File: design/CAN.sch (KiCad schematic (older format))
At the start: 4 parts, among them U4 TJA1051TK3

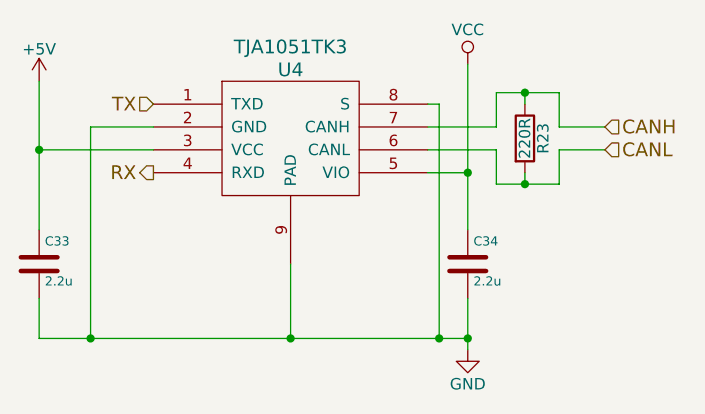
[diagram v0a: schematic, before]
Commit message: initial commit
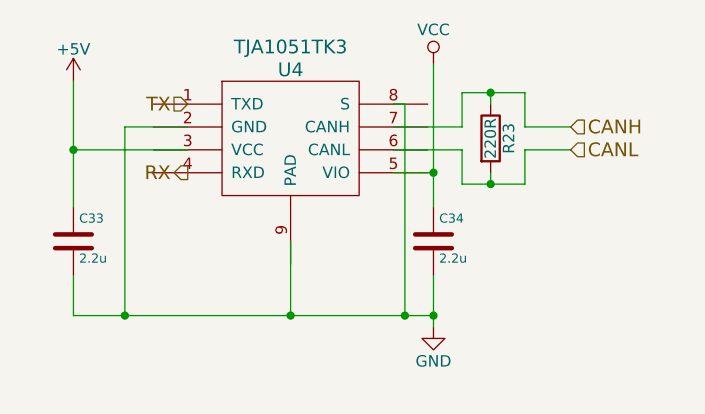
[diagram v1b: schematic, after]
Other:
- moved on the sheet: C33, C34, R23
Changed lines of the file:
@@
 LIBS:valves
 LIBS:crf_1
+LIBS:crf_2
 LIBS:VESC_6-cache
 EELAYER 25 0
@@
 L C C33
 U 1 1 53F59FA3
-P 4900 4550
-F 0 "C33" H 4925 4650 40  0000 L CNN
-F 1 "2.2u" H 4925 4475 40  0000 L CNN
-F 2 "CRF1:SMD-0603_c" H 4938 4400 30  0001 C CNN
-F 3 "" H 4900 4550 60  0000 C CNN
-	1    4900 4550
+P 5050 4450
+F 0 "C33" H 5075 4550 40  0000 L CNN
+F 1 "2.2u" H 5075 4375 40  0000 L CNN
+F 2 "CRF1:SMD-0603_c" H 5088 4300 30  0001 C CNN
+F 3 "" H 5050 4450 60  0000 C CNN
+	1    5050 4450
 	1    0    0    -1
 $EndComp
-Text HLabel 5400 4150 0    60   Output ~ 0
+Text HLabel 5550 4150 0    60   Output ~ 0
 RX
-Text HLabel 5400 3850 0    60   Input ~ 0
+Text HLabel 5550 3850 0    60   Input ~ 0
 TX
-Text HLabel 7375 3950 2    60   Input ~ 0
+Text HLabel 7225 3950 2    60   Input ~ 0
 CANH
-Text HLabel 7375 4050 2    60   Input ~ 0
+Text HLabel 7225 4050 2    60   Input ~ 0
 CANL
 $Comp
@@
 L C C34
 U 1 1 5A8B2DCC
-P 6775 4550
-F 0 "C34" H 6800 4650 40  0000 L CNN
-F 1 "2.2u" H 6800 4475 40  0000 L CNN
-F 2 "CRF1:SMD-0603_c" H 6813 4400 30  0001 C CNN
-F 3 "" H 6775 4550 60  0000 C CNN
-	1    6775 4550
+P 6625 4450
+F 0 "C34" H 6650 4550 40  0000 L CNN
+F 1 "2.2u" H 6650 4375 40  0000 L CNN
+F 2 "CRF1:SMD-0603_c" H 6663 4300 30  0001 C CNN
+F 3 "" H 6625 4450 60  0000 C CNN
+	1    6625 4450
 	1    0    0    -1
 $EndComp
@@
 L +5V #PWR063
 U 1 1 5A8B3017
-P 4900 3750
-F 0 "#PWR063" H 4900 3600 50  0001 C CNN
-F 1 "+5V" H 4900 3890 50  0000 C CNN
-F 2 "" H 4900 3750 50  0001 C CNN
-F 3 "" H 4900 3750 50  0001 C CNN
-	1    4900 3750
+P 5050 3750
+F 0 "#PWR063" H 5050 3600 50  0001 C CNN
+F 1 "+5V" H 5050 3890 50  0000 C CNN
+F 2 "" H 5050 3750 50  0001 C CNN
+F 3 "" H 5050 3750 50  0001 C CNN
+	1    5050 3750
 	1    0    0    -1
 $EndComp
@@
 L R R23
 U 1 1 5A8B3269
-P 7025 4000
-F 0 "R23" V 7105 4000 50  0000 C CNN
-F 1 "220R" V 7025 4000 50  0000 C CNN
-F 2 "CRF1:SMD-0603_r" V 6955 4000 50  0001 C CNN
-F 3 "" H 7025 4000 50  0001 C CNN
-	1    7025 4000
+P 6875 4000
+F 0 "R23" V 6955 4000 50  0000 C CNN
+F 1 "220R" V 6875 4000 50  0000 C CNN
+F 2 "CRF1:SMD-0603_r" V 6805 4000 50  0001 C CNN
+F 3 "" H 6875 4000 50  0001 C CNN
+	1    6875 4000
 	1    0    0    -1
 $EndComp
@@
 L VCC #PWR064
 U 1 1 5A8B3886
-P 6775 3675
-F 0 "#PWR064" H 6775 3525 50  0001 C CNN
-F 1 "VCC" H 6775 3825 50  0000 C CNN
-F 2 "" H 6775 3675 50  0001 C CNN
-F 3 "" H 6775 3675 50  0001 C CNN
-	1    6775 3675
+P 6625 3675
+F 0 "#PWR064" H 6625 3525 50  0001 C CNN
+F 1 "VCC" H 6625 3825 50  0000 C CNN
+F 2 "" H 6625 3675 50  0001 C CNN
+F 3 "" H 6625 3675 50  0001 C CNN
+	1    6625 3675
+	1    0    0    -1
+$EndComp
+$Comp
+L GND #PWR065
+U 1 1 5A8B3BF5
+P 6625 4825
+F 0 "#PWR065" H 6625 4575 50  0001 C CNN
+F 1 "GND" H 6625 4675 50  0000 C CNN
+F 2 "" H 6625 4825 50  0001 C CNN
+F 3 "" H 6625 4825 50  0001 C CNN
+	1    6625 4825
 	1    0    0    -1
 $EndComp
 Wire Wire Line
-	6900 4200 6900 4050
+	6750 4200 6750 4050
 Wire Wire Line
-	6900 4050 6600 4050
+	6750 4050 6450 4050
 Wire Wire Line
-	6600 3950 6900 3950
+	6450 3950 6750 3950
 Wire Wire Line
-	6900 3950 6900 3800
+	6750 3950 6750 3800
 Wire Wire Line
-	6900 3800 7175 3800
+	6750 3800 7025 3800
 Wire Wire Line
-	6600 4150 6775 4150
+	6450 4150 6625 4150
 Wire Wire Line
-	6775 3675 6775 4400
+	6625 3675 6625 4300
 Wire Wire Line
-	6775 4700 6775 4925
+	6625 4600 6625 4825
 Wire Wire Line
-	4900 4875 6775 4875
+	6000 4775 6000 4450
+Connection ~ 6000 4775
 Wire Wire Line
-	5125 4875 5125 3950
+	5275 3950 5550 3950
 Wire Wire Line
-	6000 4550 6000 4875
-Connection ~ 6000 4875
+	5050 4600 5050 4775
+Connection ~ 5275 4775
 Wire Wire Line
-	5125 3950 5400 3950
+	5050 4050 5550 4050
+Connection ~ 5050 4050
 Wire Wire Line
-	4900 4700 4900 4875
-Connection ~ 5125 4875
+	6450 3850 6500 3850
 Wire Wire Line
-	4900 3750 4900 4400
+	6500 4775 6500 3850
+Connection ~ 6500 4775
 Wire Wire Line
-	4900 4050 5400 4050
-Connection ~ 4900 4050
+	6875 3850 6875 3800
+Connection ~ 6875 3800
 Wire Wire Line
-	6600 3850 6650 3850
+	6875 4150 6875 4200
+Connection ~ 6875 4200
 Wire Wire Line
-	6650 3850 6650 4875
-Connection ~ 6650 4875
+	7025 4200 7025 4050
 Wire Wire Line
-	7025 3850 7025 3800
-Connection ~ 7025 3800
+	7025 4050 7225 4050
 Wire Wire Line
-	7025 4150 7025 4200
-Connection ~ 7025 4200
+	7025 3800 7025 3950
 Wire Wire Line
-	7175 4200 7175 4050
+	7025 3950 7225 3950
 Wire Wire Line
-	7175 4050 7375 4050
+	6750 4200 7025 4200
+Connection ~ 6625 4150
+Connection ~ 6625 4775
 Wire Wire Line
-	7175 3800 7175 3950
+	5050 4775 6625 4775
 Wire Wire Line
-	7175 3950 7375 3950
+	5050 3750 5050 4300
 Wire Wire Line
-	6900 4200 7175 4200
-Connection ~ 6775 4150
-$Comp
-L GND #PWR065
-U 1 1 5A8B3BF5
-P 6775 4925
-F 0 "#PWR065" H 6775 4675 50  0001 C CNN
-F 1 "GND" H 6775 4775 50  0000 C CNN
-F 2 "" H 6775 4925 50  0001 C CNN
-F 3 "" H 6775 4925 50  0001 C CNN
-	1    6775 4925
-	1    0    0    -1
-$EndComp
-Connection ~ 6775 4875
+	5275 3950 5275 4775
 $EndSCHEMATC

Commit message: initial commit
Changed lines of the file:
@@
 LIBS:valves
 LIBS:crf_1
-LIBS:crf_2
 LIBS:VESC_6-cache
 EELAYER 25 0
@@
 	6450 3850 6500 3850
 Wire Wire Line
-	6500 4775 6500 3850
+	6500 3850 6500 4775
 Connection ~ 6500 4775
 Wire Wire Line
